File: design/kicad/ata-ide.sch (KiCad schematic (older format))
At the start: 29 parts, among them J1 Conn_02x32_Odd_Even, J2 Conn_02x20_Odd_Even, Q1 2N2907, U1 16V8, U2 ATF750, U3 74HCT241, U4 74HCT245, U5 74HCT245

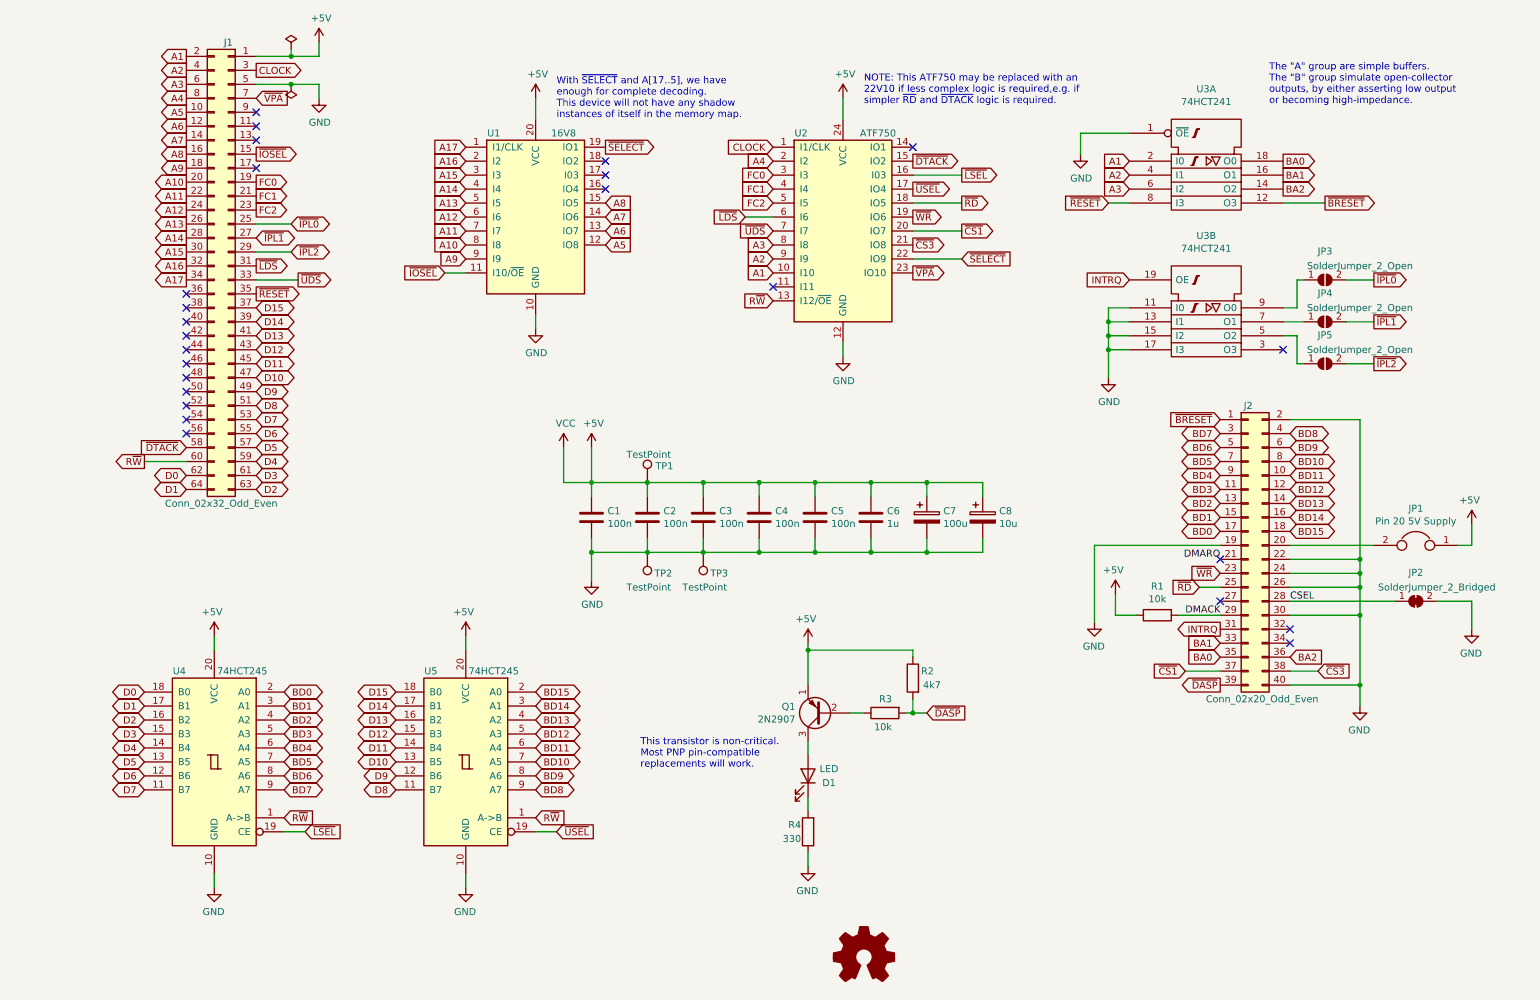
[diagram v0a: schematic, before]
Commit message: Update for version 1.1.
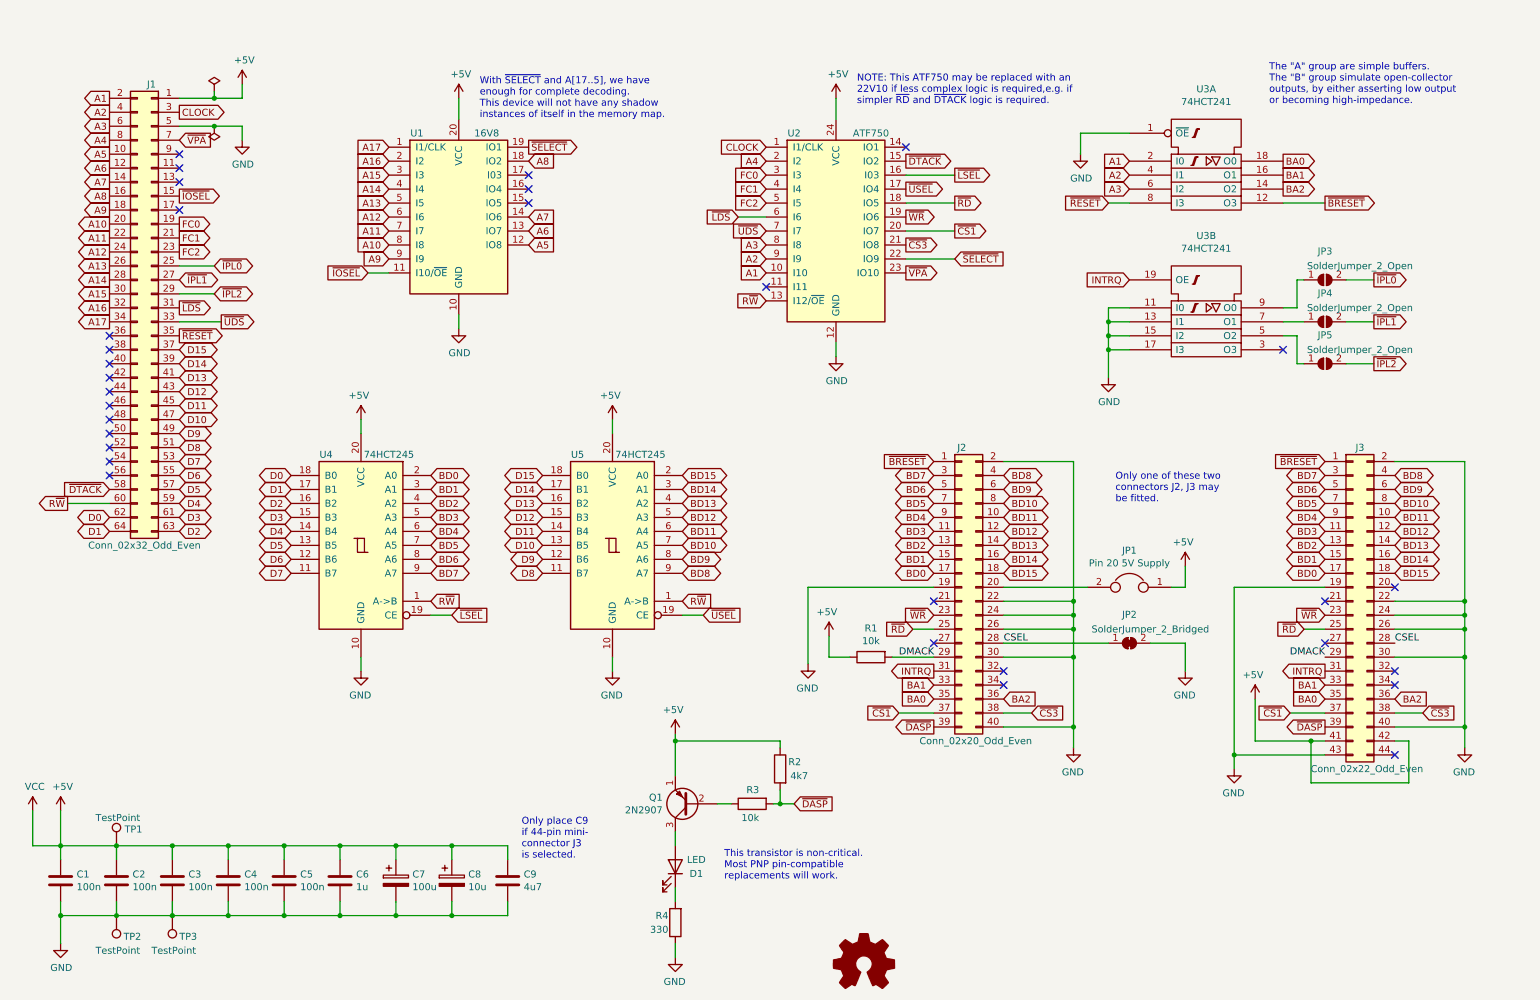
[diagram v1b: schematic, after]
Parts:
- added C9: 4u7, Capacitors_THT:C_Rect_L7.0mm_W4.5mm_P5.00mm, symbol Device:C
- added J3: Conn_02x22_Odd_Even, Pin_Headers:Pin_Header_Straight_2x22_Pitch2.00mm, symbol Connector_Generic:Conn_02x22_Odd_Even
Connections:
- net +5V: now also C9.1, J3.41 (Pin_41), J3.42 (Pin_42)
- net A8: now also U1.18 (IO2); no longer U1.15 (IO5)
- net BA0: now also J3.35 (Pin_35)
- net BA1: now also J3.33 (Pin_33)
- net BA2: now also J3.36 (Pin_36)
- net BD0: now also J3.17 (Pin_17)
- net BD1: now also J3.15 (Pin_15)
- net BD10: now also J3.8 (Pin_8)
- net BD11: now also J3.10 (Pin_10)
- net BD12: now also J3.12 (Pin_12)
- net BD13: now also J3.14 (Pin_14)
- net BD14: now also J3.16 (Pin_16)
- net BD15: now also J3.18 (Pin_18)
- net BD2: now also J3.13 (Pin_13)
- net BD3: now also J3.11 (Pin_11)
- net BD4: now also J3.9 (Pin_9)
- net BD5: now also J3.7 (Pin_7)
- net BD6: now also J3.5 (Pin_5)
- net BD7: now also J3.3 (Pin_3)
- net BD8: now also J3.4 (Pin_4)
- net BD9: now also J3.6 (Pin_6)
- net CSEL: now also J3.28 (Pin_28)
- net DMACK: now also J3.29 (Pin_29)
- net GND: now also C9.2, J3.19 (Pin_19), J3.2 (Pin_2), J3.22 (Pin_22), J3.24 (Pin_24), J3.26 (Pin_26), J3.30 (Pin_30), J3.40 (Pin_40), J3.43 (Pin_43)
- net INTRQ: now also J3.31 (Pin_31)
- net ~BRESET~: now also J3.1 (Pin_1)
- net ~CS1~: now also J3.37 (Pin_37)
- net ~CS3~: now also J3.38 (Pin_38)
- net ~DASP~: now also J3.39 (Pin_39)
- net ~RD~: now also J3.25 (Pin_25)
- net ~WR~: now also J3.23 (Pin_23)
- net DMARQ: no longer names the net of J2.21 (Pin_21)
- no-connect marks 25 -> 31
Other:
- note added: "Only one of these two\nconnectors J2, J3 may\nbe fitted."
- note added: "Only place C9\nif 44-pin mini-\nconnector J3\nis selected."
- moved on the sheet: C1, C2, C3, C4, C5, C6, C7, C8, D1, J1, J2, JP1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
